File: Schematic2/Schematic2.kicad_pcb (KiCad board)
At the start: 2 copper layers, 100 x 119 mm, 52 parts, among them SW1 Rotary_Encoder_Switch, U1 Kailhlowprofile, U10 Kailhlowprofile, U11 Kailhlowprofile, U12 Kailhlowprofile, U13 Kailhlowprofile, U14 Kailhlowprofile, U15 Kailhlowprofile, U16 Kailhlowprofile, U17 Kailhlowprofile, U18 Kailhlowprofile, U19 Kailhlowprofile, U2 Kailhlowprofile, U20 Kailhlowprofile, U3 Kailhlowprofile, U4 Kailhlowprofile, U5 Kailhlowprofile, U6 Kailhlowprofile, U7 Kailhlowprofile, U8 Kailhlowprofile, U9 Kailhlowprofile

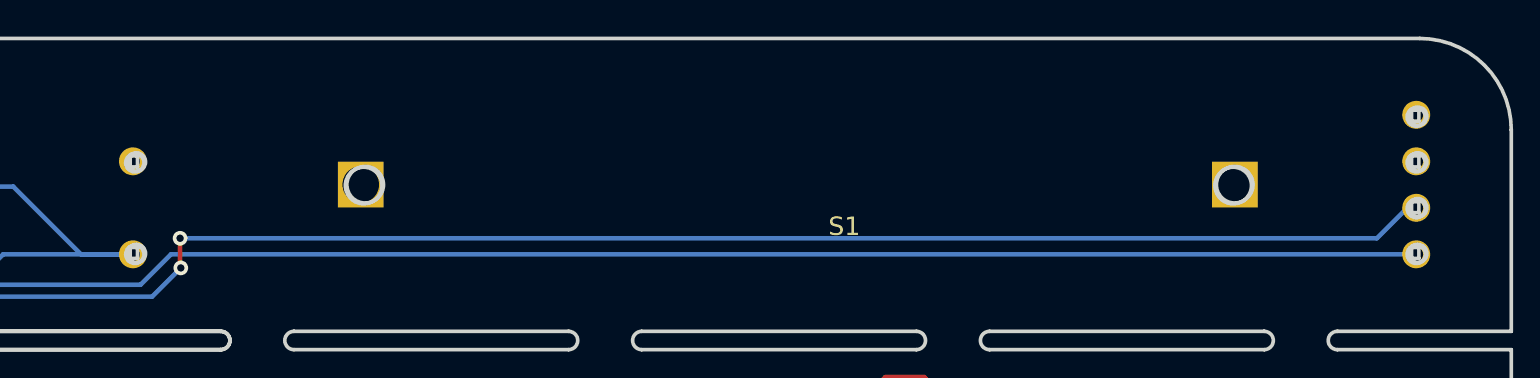
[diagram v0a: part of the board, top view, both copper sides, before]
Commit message: THE FINAL
urgh. Last and final PCB
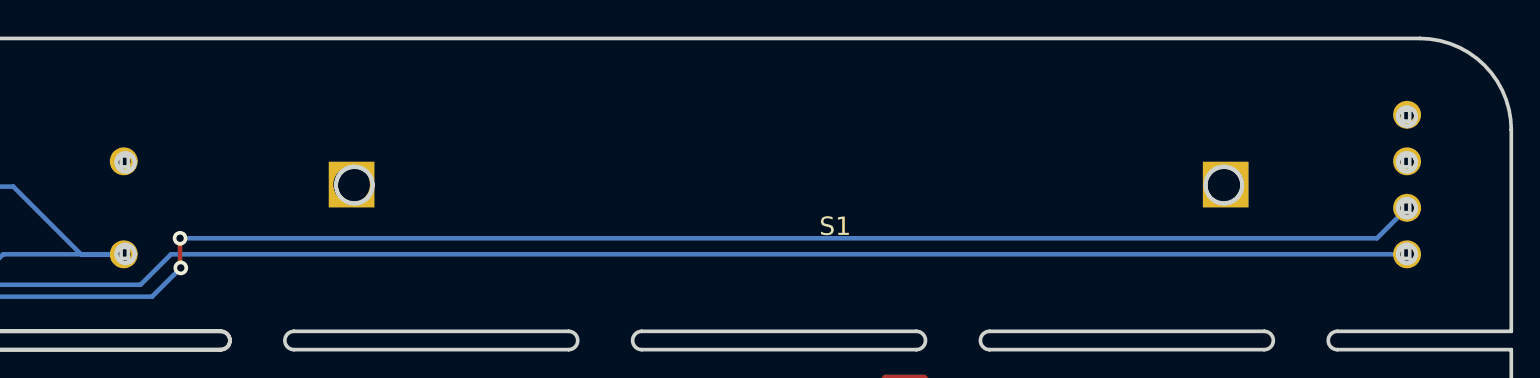
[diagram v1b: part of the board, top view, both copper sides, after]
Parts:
- moved S1 0.50 mm to (235.6, 25.8)
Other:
- outline, holes or cut-outs redrawn
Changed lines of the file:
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@@
   )
   (module alps_slider:ALPS-Slider (layer F.Cu)
-    (at 236.1184 25.8064 180)
+    (at 235.6184 25.8064 180)
     (fp_text reference S1 (at -6.858 -2.286 180) (layer F.SilkS)
       (effects (font (size 1 1) (thickness 0.15)))
@@
   (gr_line (start 242.311999 89.299) (end 241.511999 89.299) (layer Edge.Cuts) (width 0.2))
   (gr_circle (center 252.411999 105.324) (end 253.312 105.324) (layer Edge.Cuts) (width 0.2))
-  (gr_circle (center 204.302975 24.573999) (end 204.802975 24.573999) (layer Edge.Cuts) (width 0.2))
+  (gr_circle (center 203.702975 24.573999) (end 204.202975 24.573999) (layer Edge.Cuts) (width 0.2))
   (gr_line (start 194.411999 110.324) (end 194.411999 117.824) (layer Edge.Cuts) (width 0.2))
   (gr_arc (start 193.911999 110.324) (end 194.411999 110.324) (angle -180) (layer Edge.Cuts) (width 0.2))
@@
   (gr_line (start 193.412 91.324) (end 193.412 106.324) (layer Edge.Cuts) (width 0.2))
   (gr_line (start 188.962 32.423999) (end 186.862 32.423999) (layer Edge.Cuts) (width 0.2))
-  (gr_circle (center 274.302975 27.073999) (end 274.802975 27.073999) (layer Edge.Cuts) (width 0.2))
+  (gr_circle (center 273.702975 27.073999) (end 274.202975 27.073999) (layer Edge.Cuts) (width 0.2))
   (gr_circle (center 186.662 111.723999) (end 187.162 111.723999) (layer Edge.Cuts) (width 0.2))
   (gr_circle (center 195.411999 25.823999) (end 195.911999 25.823999) (layer Edge.Cuts) (width 0.2))
-  (gr_circle (center 204.302975 29.573999) (end 204.802975 29.573999) (layer Edge.Cuts) (width 0.2))
-  (gr_circle (center 264.302975 25.814975) (end 265.302975 25.814975) (layer Edge.Cuts) (width 0.2))
+  (gr_circle (center 203.702975 29.573999) (end 204.202975 29.573999) (layer Edge.Cuts) (width 0.2))
+  (gr_circle (center 263.702975 25.814975) (end 264.702975 25.814975) (layer Edge.Cuts) (width 0.2))
   (gr_line (start 186.862 32.423999) (end 186.862 30.423999) (layer Edge.Cuts) (width 0.2))
   (gr_line (start 186.862 30.423999) (end 188.962 30.423999) (layer Edge.Cuts) (width 0.2))
@@
   (gr_line (start 194.411999 72.324) (end 194.411999 87.324) (layer Edge.Cuts) (width 0.2))
   (gr_arc (start 193.911999 106.324) (end 193.412 106.324) (angle -180) (layer Edge.Cuts) (width 0.2))
-  (gr_circle (center 274.302975 24.573999) (end 274.802975 24.573999) (layer Edge.Cuts) (width 0.2))
+  (gr_circle (center 273.702975 24.573999) (end 274.202975 24.573999) (layer Edge.Cuts) (width 0.2))
   (gr_circle (center 180.912 23.323999) (end 181.412 23.323999) (layer Edge.Cuts) (width 0.2))
   (gr_circle (center 189.162 111.723999) (end 189.662 111.723999) (layer Edge.Cuts) (width 0.2))
-  (gr_circle (center 216.802975 25.814975) (end 217.802975 25.814975) (layer Edge.Cuts) (width 0.2))
+  (gr_circle (center 216.202975 25.814975) (end 217.202975 25.814975) (layer Edge.Cuts) (width 0.2))
   (gr_arc (start 274.412 131.823999) (end 274.412 136.823999) (angle -90) (layer Edge.Cuts) (width 0.2))
   (gr_line (start 279.412 111.824) (end 279.412 131.823999) (layer Edge.Cuts) (width 0.2))
@@
   (gr_line (start 179.412 22.823999) (end 179.412 111.823999) (layer Edge.Cuts) (width 0.2))
   (gr_circle (center 195.411999 28.323999) (end 195.911999 28.323999) (layer Edge.Cuts) (width 0.2))
-  (gr_circle (center 274.302975 29.573999) (end 274.802975 29.573999) (layer Edge.Cuts) (width 0.2))
+  (gr_circle (center 273.702975 29.573999) (end 274.202975 29.573999) (layer Edge.Cuts) (width 0.2))
   (gr_circle (center 184.162 41.723999) (end 184.662 41.723999) (layer Edge.Cuts) (width 0.2))
-  (gr_circle (center 274.302975 22.073999) (end 274.802975 22.073999) (layer Edge.Cuts) (width 0.2))
+  (gr_circle (center 273.702975 22.073999) (end 274.202975 22.073999) (layer Edge.Cuts) (width 0.2))
   (gr_circle (center 262.411999 65.324) (end 263.311999 65.324) (layer Edge.Cuts) (width 0.2))
   (gr_circle (center 262.411999 85.324) (end 263.311999 85.324) (layer Edge.Cuts) (width 0.2))
